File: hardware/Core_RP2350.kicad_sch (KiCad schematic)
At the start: 76 parts, among them J19 Micro_SD_Card_Det_Hirose_DM3AT, J20 USB_C_Receptacle_USB2.0, J21 5-146281-3, J22 5-146281-3, J4 AudioJack3, SW1 SPST-NO, SW2 SPST-NO, SW3 SPST-NO, U1 RP2350B-QFN80, U2 ADUM4160, U3 W25Q128JVS

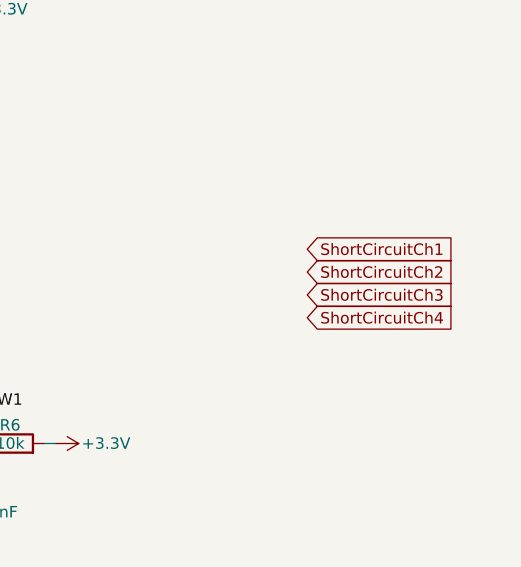
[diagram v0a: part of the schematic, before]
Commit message: draft split rail power supply design
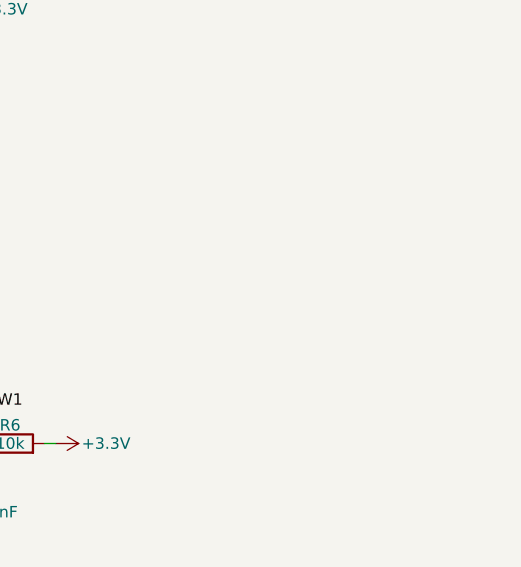
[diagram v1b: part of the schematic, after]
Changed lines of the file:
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@@
-		)
-	)
-	(global_label "ShortCircuitCh1"
-		(shape input)
-		(at 299.72 81.28 0)
-		(fields_autoplaced yes)
-		(effects
-			(font
-				(size 1.27 1.27)
-			)
-			(justify left)
-		)
-		(property "Intersheetrefs" "${INTERSHEET_REFS}"
-			(at 317.5822 81.28 0)
-			(effects
-				(font
-					(size 1.27 1.27)
-				)
-				(justify left)
-				(hide yes)
-			)
 		)
 	)
@@
 		)
 	)
-	(global_label "ShortCircuitCh3"
-		(shape input)
-		(at 299.72 86.36 0)
-		(fields_autoplaced yes)
-		(effects
-			(font
-				(size 1.27 1.27)
-			)
-			(justify left)
-		)
-		(property "Intersheetrefs" "${INTERSHEET_REFS}"
-			(at 317.5822 86.36 0)
-			(effects
-				(font
-					(size 1.27 1.27)
-				)
-				(justify left)
-				(hide yes)
-			)
-		)
-	)
-	(global_label "ShortCircuitCh4"
-		(shape input)
-		(at 299.72 88.9 0)
-		(fields_autoplaced yes)
-		(effects
-			(font
-				(size 1.27 1.27)
-			)
-			(justify left)
-		)
-		(property "Intersheetrefs" "${INTERSHEET_REFS}"
-			(at 317.5822 88.9 0)
-			(effects
-				(font
-					(size 1.27 1.27)
-				)
-				(justify left)
-				(hide yes)
-			)
-		)
-	)
 	(global_label "DAC_2_CS"
 		(shape input)
@@
 			(effects
 				(font
-					(size 1.27 1.27)
-				)
-				(justify left)
-				(hide yes)
-			)
-		)
-	)
-	(global_label "ShortCircuitCh2"
-		(shape input)
-		(at 299.72 83.82 0)
-		(fields_autoplaced yes)
-		(effects
-			(font
-				(size 1.27 1.27)
-			)
-			(justify left)
-		)
-		(property "Intersheetrefs" "${INTERSHEET_REFS}"
-			(at 317.5822 83.82 0)
-			(effects
-				(font
